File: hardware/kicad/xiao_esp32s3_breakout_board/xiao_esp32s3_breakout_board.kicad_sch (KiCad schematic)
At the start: 8 parts, among them J1 XIAO_BREAKOUT_BOARD, J2 Conn_02x03_Odd_Even, J3 Conn_01x02_Pin, J4 Conn_01x07_Socket, J5 Conn_01x07_Socket, U1 XIAO-ESP32-S3

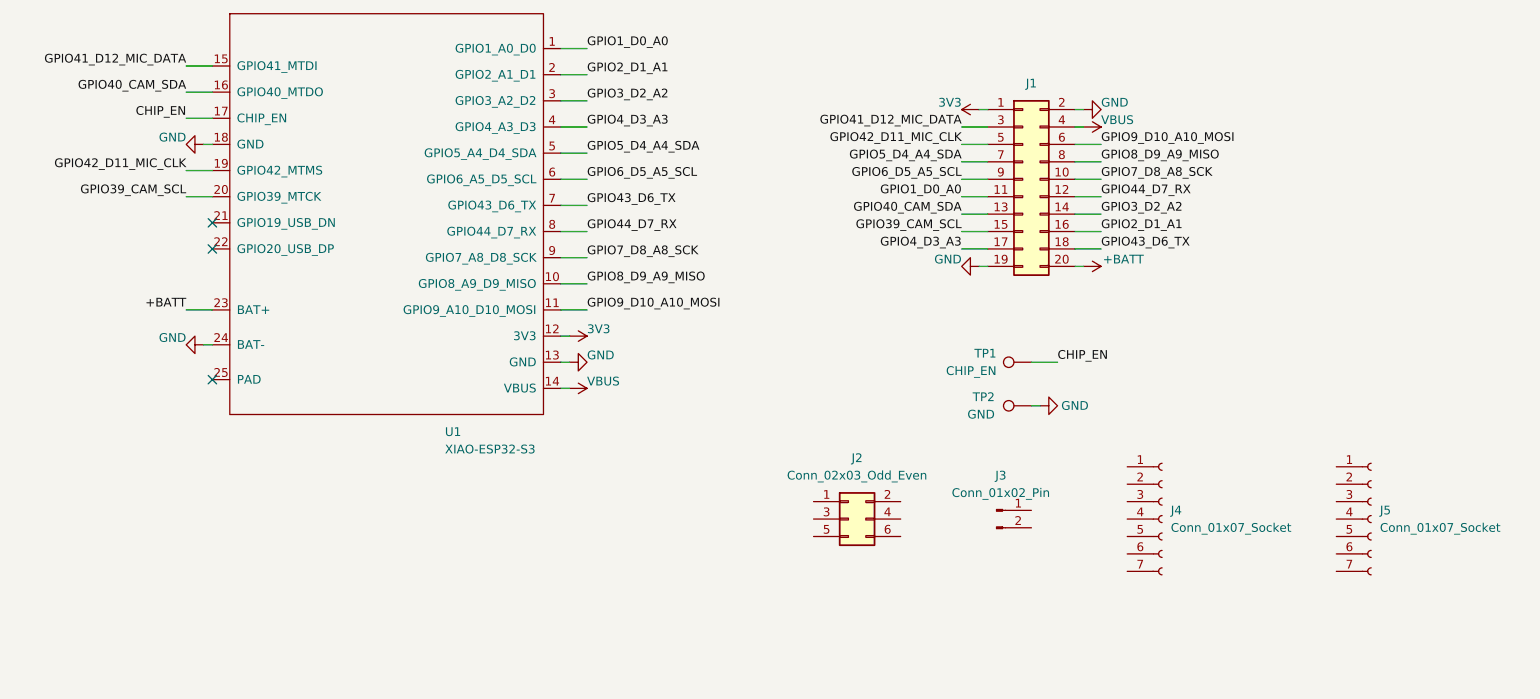
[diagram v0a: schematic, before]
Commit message: これで注文した
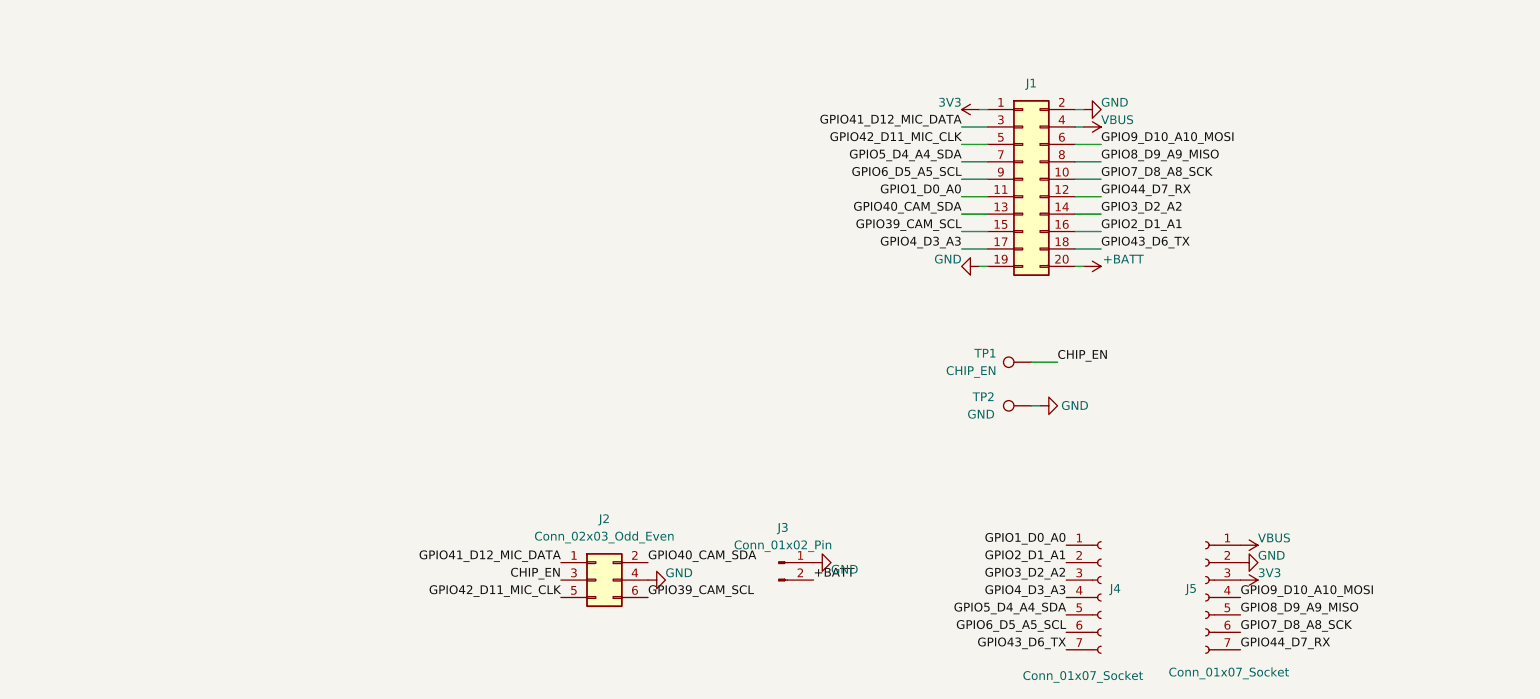
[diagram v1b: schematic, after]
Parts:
- removed U1: XIAO-ESP32-S3, @自分用:XIAO-ESP32-S3-SMD, symbol Seeed_Studio_XIAO_Series:XIAO-ESP32-S3-SMD
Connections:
- net +BATT: now also J3.2 (Pin_2)
- net 3V3: now also J5.3 (Pin_3)
- net CHIP_EN: now also J2.3 (Pin_3)
- net GND: now also J2.4 (Pin_4), J3.1 (Pin_1), J5.2 (Pin_2)
- net GPIO1_D0_A0: now also J4.1 (Pin_1)
- net GPIO2_D1_A1: now also J4.2 (Pin_2)
- net GPIO39_CAM_SCL: now also J2.6 (Pin_6)
- net GPIO3_D2_A2: now also J4.3 (Pin_3)
- net GPIO40_CAM_SDA: now also J2.2 (Pin_2)
- net GPIO41_D12_MIC_DATA: now also J2.1 (Pin_1)
- net GPIO42_D11_MIC_CLK: now also J2.5 (Pin_5)
- net GPIO43_D6_TX: now also J4.7 (Pin_7)
- net GPIO44_D7_RX: now also J5.7 (Pin_7)
- net GPIO4_D3_A3: now also J4.4 (Pin_4)
- net GPIO5_D4_A4_SDA: now also J4.5 (Pin_5)
- net GPIO6_D5_A5_SCL: now also J4.6 (Pin_6)
- net GPIO7_D8_A8_SCK: now also J5.6 (Pin_6)
- net GPIO8_D9_A9_MISO: now also J5.5 (Pin_5)
- net GPIO9_D10_A10_MOSI: now also J5.4 (Pin_4)
- net VBUS: now also J5.1 (Pin_1)
- no-connect marks 3 -> 0
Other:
- moved on the sheet: J2, J3, J4, J5
